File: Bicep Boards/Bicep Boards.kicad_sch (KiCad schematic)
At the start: 17 parts, among them J1 SM02B-SRSS-TB_LF__SN_, J11 69167-107HLF, J4 69167-107HLF, J9 87583-2010RPLF, U1 ESP32-S3-WROOM-1-N16R8, U11 TS3A5018D, U12 TS3A5018D, U4 LSM6DSMTR, U9 LP2950CZ-3.3_LFT3

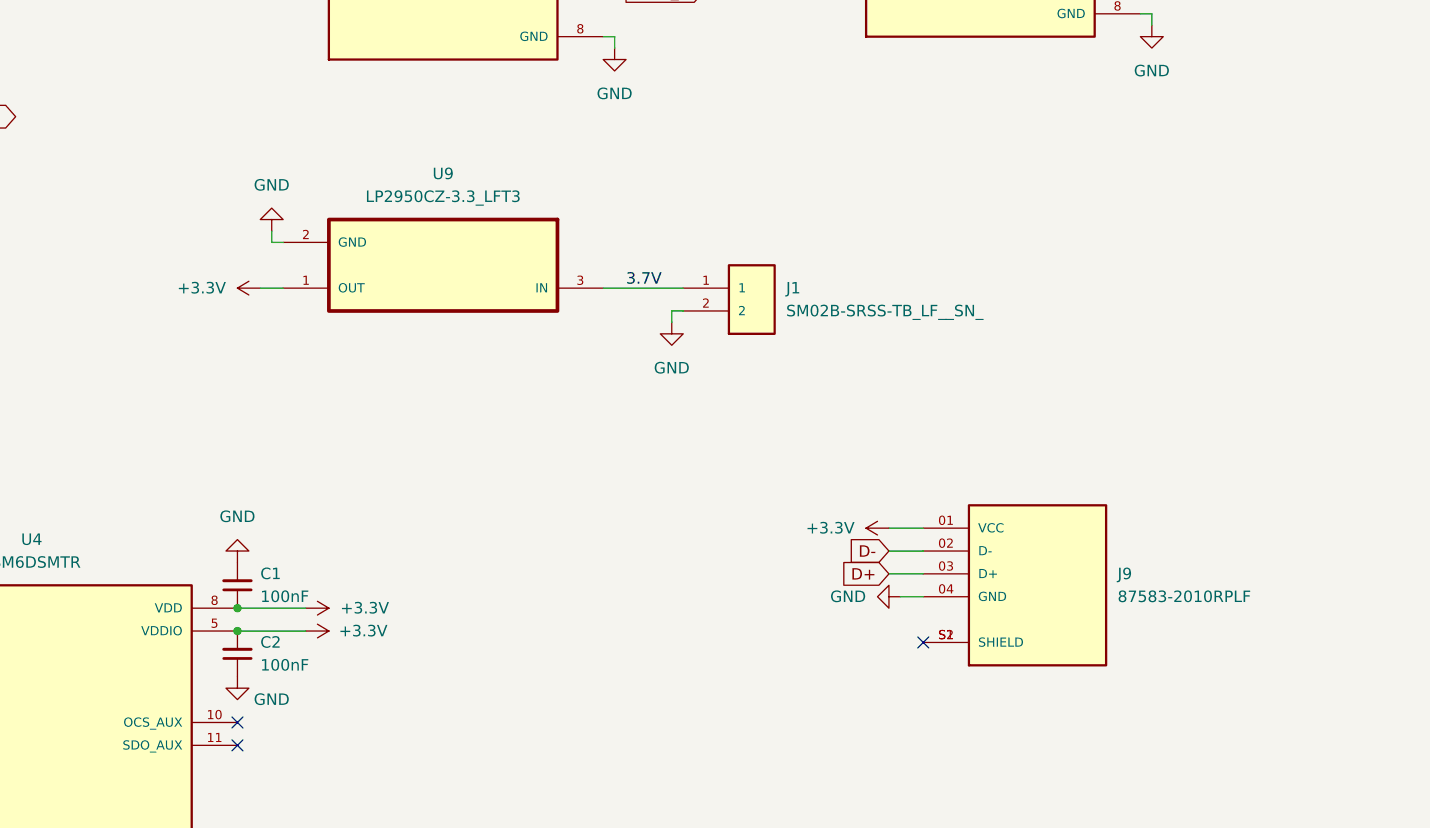
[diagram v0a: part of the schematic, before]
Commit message: Version 2
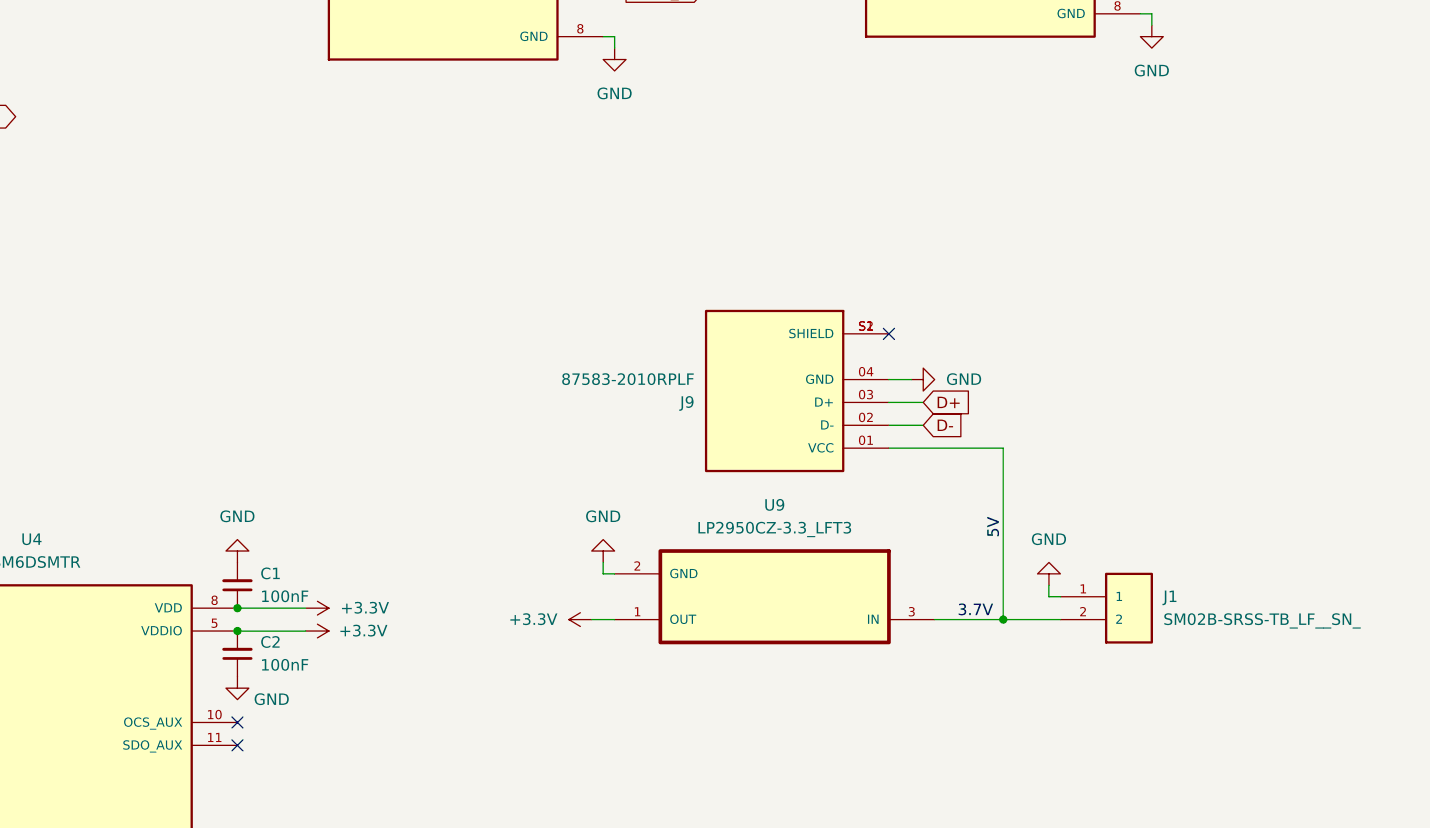
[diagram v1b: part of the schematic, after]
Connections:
- net +3.3V: no longer J9.01 (VCC)
- net 3.7V: now also J1.2, J9.01 (VCC); no longer J1.1
- net GND: now also J1.1; no longer J1.2
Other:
- moved on the sheet: J1, J9, U9
